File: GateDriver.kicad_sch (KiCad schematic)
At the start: 11 parts, among them U4 IR2110

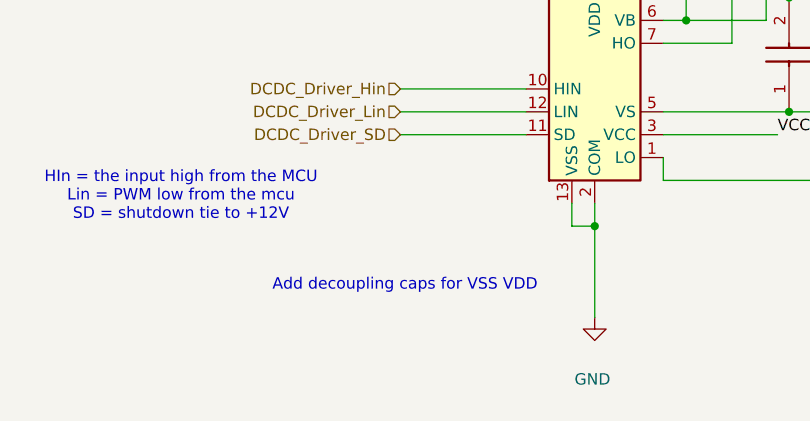
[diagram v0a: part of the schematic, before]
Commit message: Autosave
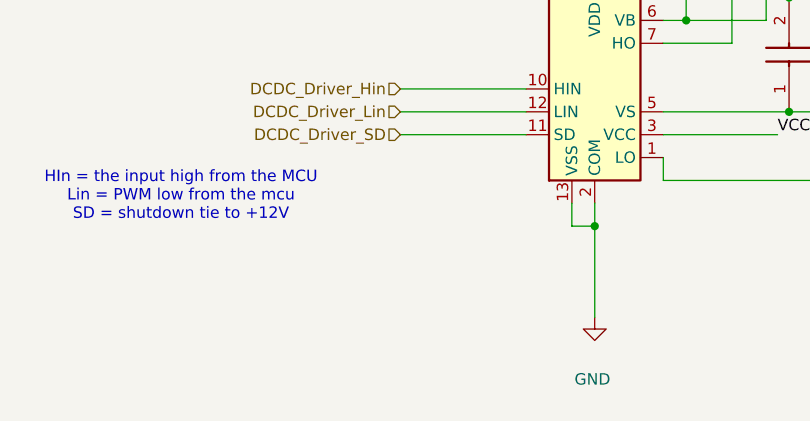
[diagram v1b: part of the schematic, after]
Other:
- note removed: "Add decoupling caps for VSS VDD"
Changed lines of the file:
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@@
 	(generator_version "10.0")
 	(paper "A4")
-	(text "Add decoupling caps for VSS VDD"
-		(exclude_from_sim no)
-		(at 61.468 80.264 0)
-		(effects
-			(font
-				(size 1.27 1.27)
-			)
-		)
-	)
 	(text "HIn = the input high from the MCU\nLin = PWM low from the mcu\nSD = shutdown tie to +12V"
 		(exclude_from_sim no)
